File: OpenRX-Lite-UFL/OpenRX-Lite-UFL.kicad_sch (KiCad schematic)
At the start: 0 parts

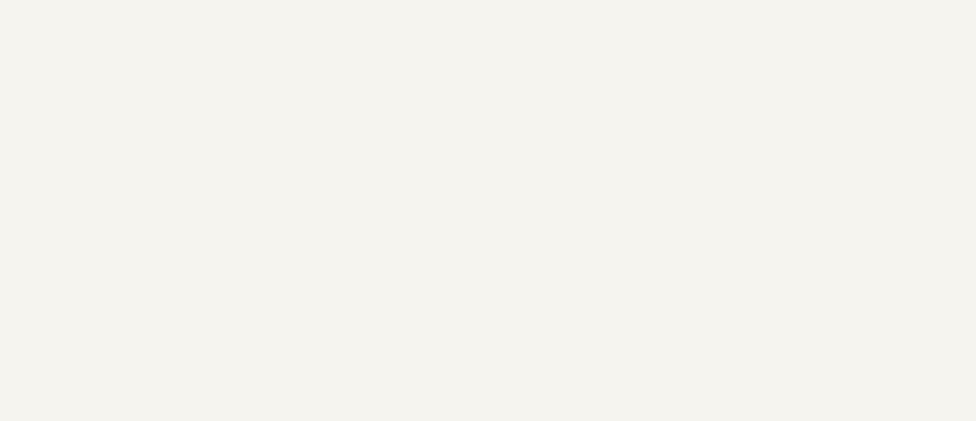
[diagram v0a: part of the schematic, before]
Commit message: annotate
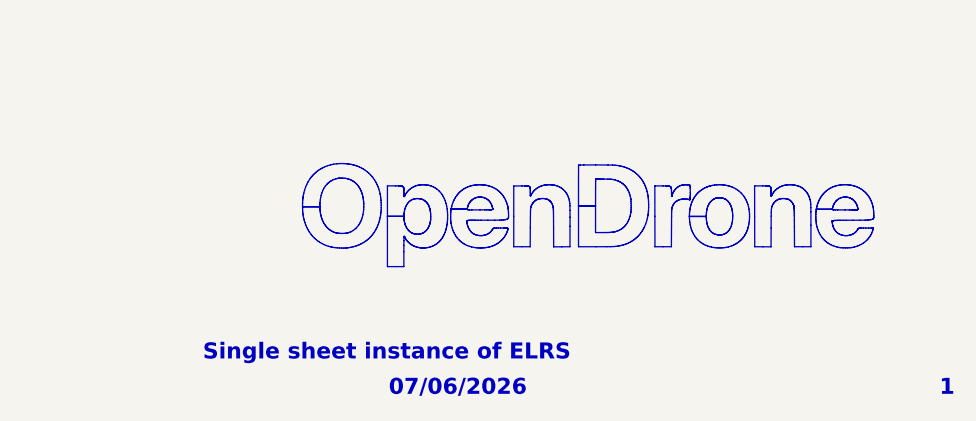
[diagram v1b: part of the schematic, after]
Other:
- note added: "07/06/2026"
- note added: "1"
- note added: "Single sheet instance of ELRS"
